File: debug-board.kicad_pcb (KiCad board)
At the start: 2 copper layers, 10 parts, among them P1 CONN_01X04, P2 CONN_01X01

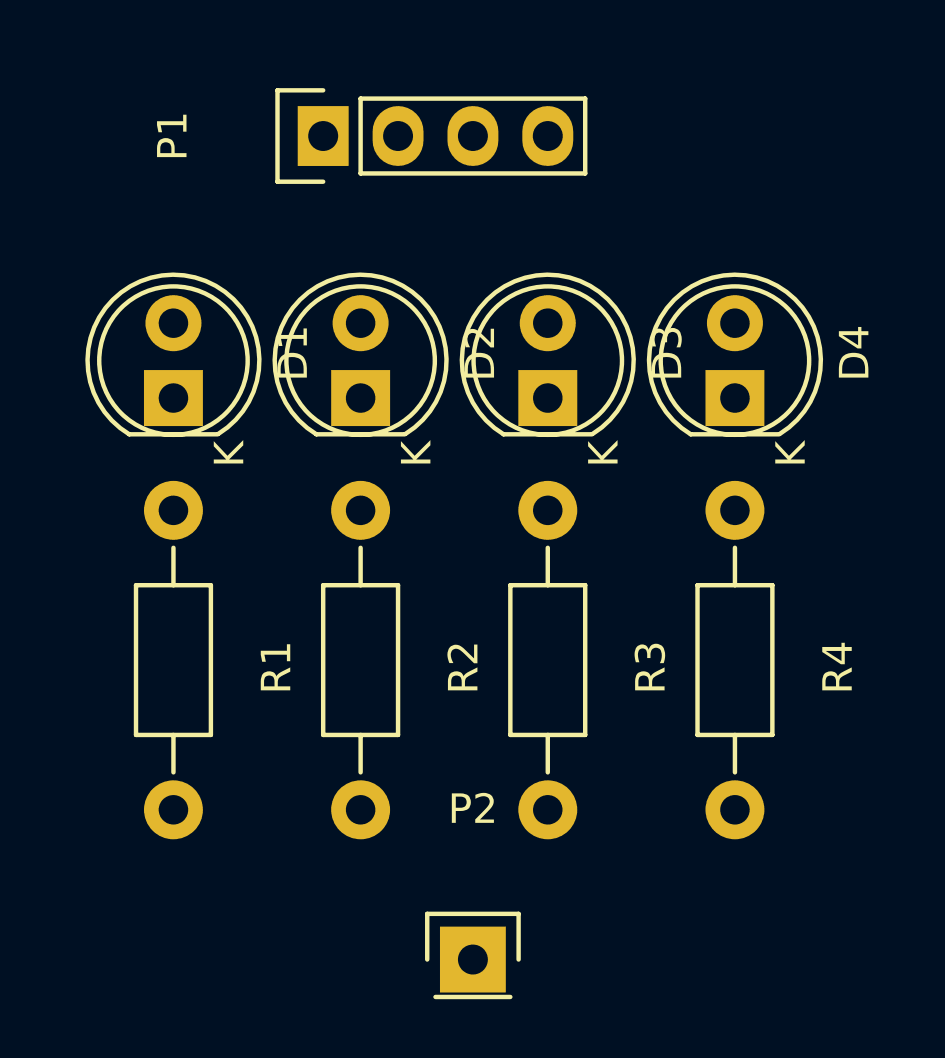
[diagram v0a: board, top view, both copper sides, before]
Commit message: Layout PCB.
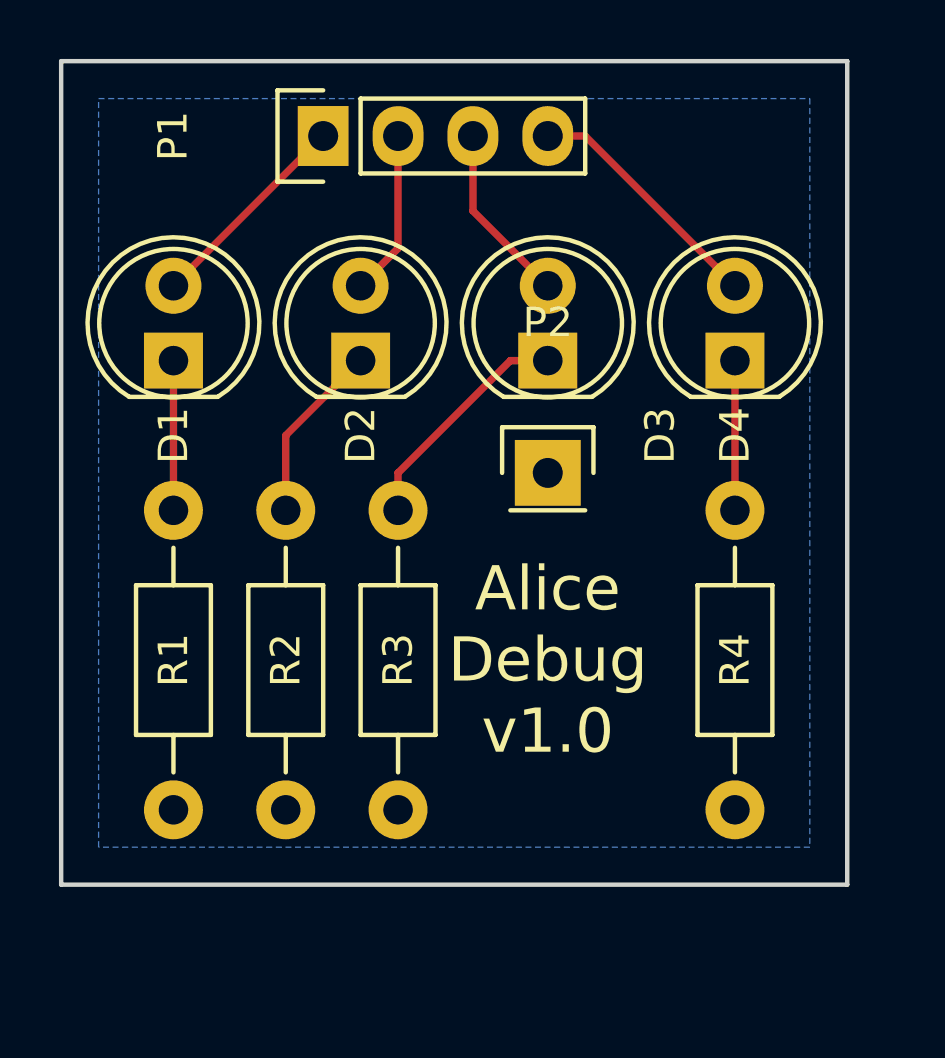
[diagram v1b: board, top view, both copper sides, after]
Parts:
- moved P2 16.7 mm to (151.1, 101.6)
- moved R3 5.08 mm to (146.1, 108.0)
- moved R2 2.54 mm to (142.2, 108.0)
- moved D1 1.27 mm to (138.4, 97.8)
- moved D2 1.27 mm to (144.8, 97.8)
- moved D3 1.27 mm to (151.1, 97.8)
- moved D4 1.27 mm to (157.5, 97.8)
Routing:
- net Net-(D4-Pad2): track 0.00 -> 8.45 mm
- net Net-(D3-Pad1): track 0.00 -> 7.93 mm
- net Net-(D1-Pad2): track 0.00 -> 7.18 mm
- net Net-(D2-Pad1): track 0.00 -> 6.13 mm
- net Net-(D3-Pad2): track 0.00 -> 6.13 mm
- net Net-(D2-Pad2): track 0.00 -> 5.61 mm
- net Net-(D4-Pad1): track 0.00 -> 5.08 mm
- net Net-(D1-Pad1): track 0.00 -> 5.08 mm
- added copper zone on B.Cu, net GND
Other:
- board outline added: 26.7 x 27.9 mm
- board text added: "Alice Debug v1.0"
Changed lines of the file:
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@@
   (general
     (links 12)
-    (no_connects 12)
+    (no_connects 0)
     (area 0 0 0 0)
     (thickness 1.6)
-    (drawings 0)
-    (tracks 0)
+    (drawings 5)
+    (tracks 14)
     (zones 0)
     (modules 10)
@@
   )
   (module LEDs:LED-5MM (layer F.Cu)
-    (at 138.43 99.06 90)
+    (at 138.43 97.79 90)
     (descr "LED 5mm round vertical")
     (tags "LED 5mm round vertical")
-    (fp_text reference D1 (at 1.524 4.064 90) (layer F.SilkS)
-      (effects (font (size 1 1) (thickness 0.15)))
-    )
-    (fp_text value LED (at 1.524 -3.937 90) (layer F.Fab)
+    (fp_text reference D1 (at -2.54 0 90) (layer F.SilkS)
+      (effects (font (size 1 1) (thickness 0.15)))
+    )
+    (fp_text value LED (at 1.524 -3.937 90) (layer F.Fab) hide
       (effects (font (size 1 1) (thickness 0.15)))
     )
@@
     (fp_line (start -1.23 1.5) (end -1.23 -1.5) (layer F.SilkS) (width 0.15))
     (fp_circle (center 1.27 0) (end 0.97 -2.5) (layer F.SilkS) (width 0.15))
-    (fp_text user K (at -1.905 1.905 90) (layer F.SilkS)
-      (effects (font (size 1 1) (thickness 0.15)))
-    )
     (pad 1 thru_hole rect (at 0 0 180) (size 2 1.9) (drill 1.00076) (layers *.Cu *.Mask F.SilkS)
       (net 1 "Net-(D1-Pad1)"))
@@
   )
   (module LEDs:LED-5MM (layer F.Cu)
-    (at 144.78 99.06 90)
+    (at 144.78 97.79 90)
     (descr "LED 5mm round vertical")
     (tags "LED 5mm round vertical")
-    (fp_text reference D2 (at 1.524 4.064 90) (layer F.SilkS)
-      (effects (font (size 1 1) (thickness 0.15)))
-    )
-    (fp_text value LED (at 1.524 -3.937 90) (layer F.Fab)
+    (fp_text reference D2 (at -2.54 0 90) (layer F.SilkS)
+      (effects (font (size 1 1) (thickness 0.15)))
+    )
+    (fp_text value LED (at 1.524 -3.937 90) (layer F.Fab) hide
       (effects (font (size 1 1) (thickness 0.15)))
     )
@@
     (fp_line (start -1.23 1.5) (end -1.23 -1.5) (layer F.SilkS) (width 0.15))
     (fp_circle (center 1.27 0) (end 0.97 -2.5) (layer F.SilkS) (width 0.15))
-    (fp_text user K (at -1.905 1.905 90) (layer F.SilkS)
-      (effects (font (size 1 1) (thickness 0.15)))
-    )
     (pad 1 thru_hole rect (at 0 0 180) (size 2 1.9) (drill 1.00076) (layers *.Cu *.Mask F.SilkS)
       (net 3 "Net-(D2-Pad1)"))
@@
   )
   (module LEDs:LED-5MM (layer F.Cu)
-    (at 151.13 99.06 90)
+    (at 151.13 97.79 90)
     (descr "LED 5mm round vertical")
     (tags "LED 5mm round vertical")
-    (fp_text reference D3 (at 1.524 4.064 90) (layer F.SilkS)
-      (effects (font (size 1 1) (thickness 0.15)))
-    )
-    (fp_text value LED (at 1.524 -3.937 90) (layer F.Fab)
+    (fp_text reference D3 (at -2.54 3.81 90) (layer F.SilkS)
+      (effects (font (size 1 1) (thickness 0.15)))
+    )
+    (fp_text value LED (at 1.524 -3.937 90) (layer F.Fab) hide
       (effects (font (size 1 1) (thickness 0.15)))
     )
@@
     (fp_line (start -1.23 1.5) (end -1.23 -1.5) (layer F.SilkS) (width 0.15))
     (fp_circle (center 1.27 0) (end 0.97 -2.5) (layer F.SilkS) (width 0.15))
-    (fp_text user K (at -1.905 1.905 90) (layer F.SilkS)
-      (effects (font (size 1 1) (thickness 0.15)))
-    )
     (pad 1 thru_hole rect (at 0 0 180) (size 2 1.9) (drill 1.00076) (layers *.Cu *.Mask F.SilkS)
       (net 5 "Net-(D3-Pad1)"))
@@
   )
   (module LEDs:LED-5MM (layer F.Cu)
-    (at 157.48 99.06 90)
+    (at 157.48 97.79 90)
     (descr "LED 5mm round vertical")
     (tags "LED 5mm round vertical")
-    (fp_text reference D4 (at 1.524 4.064 90) (layer F.SilkS)
-      (effects (font (size 1 1) (thickness 0.15)))
-    )
-    (fp_text value LED (at 1.524 -3.937 90) (layer F.Fab)
+    (fp_text reference D4 (at -2.54 0 90) (layer F.SilkS)
+      (effects (font (size 1 1) (thickness 0.15)))
+    )
+    (fp_text value LED (at 1.524 -3.937 90) (layer F.Fab) hide
       (effects (font (size 1 1) (thickness 0.15)))
     )
@@
     (fp_line (start -1.23 1.5) (end -1.23 -1.5) (layer F.SilkS) (width 0.15))
     (fp_circle (center 1.27 0) (end 0.97 -2.5) (layer F.SilkS) (width 0.15))
-    (fp_text user K (at -1.905 1.905 90) (layer F.SilkS)
-      (effects (font (size 1 1) (thickness 0.15)))
-    )
     (pad 1 thru_hole rect (at 0 0 180) (size 2 1.9) (drill 1.00076) (layers *.Cu *.Mask F.SilkS)
       (net 7 "Net-(D4-Pad1)"))
@@
       (effects (font (size 1 1) (thickness 0.15)))
     )
-    (fp_text value CONN_01X04 (at 0 -3.1 90) (layer F.Fab)
+    (fp_text value CONN_01X04 (at 0 -3.1 90) (layer F.Fab) hide
       (effects (font (size 1 1) (thickness 0.15)))
     )
@@
   )
   (module Pin_Headers:Pin_Header_Straight_1x01 (layer F.Cu)
-    (at 148.59 118.11)
+    (at 151.13 101.6)
     (descr "Through hole pin header")
     (tags "pin header")
@@
       (effects (font (size 1 1) (thickness 0.15)))
     )
-    (fp_text value CONN_01X01 (at 0 -3.1) (layer F.Fab)
+    (fp_text value CONN_01X01 (at 0 -3.1) (layer F.Fab) hide
       (effects (font (size 1 1) (thickness 0.15)))
     )
@@
     (descr "Resistor, Axial,  RM 10mm, 1/3W,")
     (tags "Resistor, Axial, RM 10mm, 1/3W,")
-    (fp_text reference R1 (at 0.24892 -3.50012 270) (layer F.SilkS)
-      (effects (font (size 1 1) (thickness 0.15)))
-    )
-    (fp_text value 220 (at 3.81 3.81 270) (layer F.Fab)
+    (fp_text reference R1 (at 0 0 270) (layer F.SilkS)
+      (effects (font (size 1 1) (thickness 0.15)))
+    )
+    (fp_text value 220 (at 3.81 3.81 270) (layer F.Fab) hide
       (effects (font (size 1 1) (thickness 0.15)))
     )
@@
   )
   (module Resistors_ThroughHole:Resistor_Horizontal_RM10mm (layer F.Cu)
-    (at 144.78 107.95 270)
+    (at 142.24 107.95 270)
     (descr "Resistor, Axial,  RM 10mm, 1/3W,")
     (tags "Resistor, Axial, RM 10mm, 1/3W,")
-    (fp_text reference R2 (at 0.24892 -3.50012 270) (layer F.SilkS)
-      (effects (font (size 1 1) (thickness 0.15)))
-    )
-    (fp_text value 220 (at 3.81 3.81 270) (layer F.Fab)
+    (fp_text reference R2 (at 0 0 270) (layer F.SilkS)
+      (effects (font (size 1 1) (thickness 0.15)))
+    )
+    (fp_text value 220 (at 3.81 3.81 270) (layer F.Fab) hide
       (effects (font (size 1 1) (thickness 0.15)))
     )
@@
   )
   (module Resistors_ThroughHole:Resistor_Horizontal_RM10mm (layer F.Cu)
-    (at 151.13 107.95 270)
+    (at 146.05 107.95 270)
     (descr "Resistor, Axial,  RM 10mm, 1/3W,")
     (tags "Resistor, Axial, RM 10mm, 1/3W,")
-    (fp_text reference R3 (at 0.24892 -3.50012 270) (layer F.SilkS)
-      (effects (font (size 1 1) (thickness 0.15)))
-    )
-    (fp_text value 220 (at 3.81 3.81 270) (layer F.Fab)
+    (fp_text reference R3 (at 0 0 270) (layer F.SilkS)
+      (effects (font (size 1 1) (thickness 0.15)))
+    )
+    (fp_text value 220 (at 3.81 3.81 270) (layer F.Fab) hide
       (effects (font (size 1 1) (thickness 0.15)))
     )
@@
     (descr "Resistor, Axial,  RM 10mm, 1/3W,")
     (tags "Resistor, Axial, RM 10mm, 1/3W,")
-    (fp_text reference R4 (at 0.24892 -3.50012 270) (layer F.SilkS)
-      (effects (font (size 1 1) (thickness 0.15)))
-    )
-    (fp_text value 220 (at 3.81 3.81 270) (layer F.Fab)
+    (fp_text reference R4 (at 0 0 270) (layer F.SilkS)
+      (effects (font (size 1 1) (thickness 0.15)))
+    )
+    (fp_text value 220 (at 3.81 3.81 270) (layer F.Fab) hide
       (effects (font (size 1 1) (thickness 0.15)))
     )
@@
     )
   )
+  (gr_text "Alice\nDebug\nv1.0" (at 151.13 107.95) (layer F.SilkS)
+    (effects (font (size 1.5 1.5) (thickness 0.3)))
+  )
+  (gr_line (start 134.62 115.57) (end 134.62 87.63) (angle 90) (layer Edge.Cuts) (width 0.15))
+  (gr_line (start 161.29 115.57) (end 134.62 115.57) (angle 90) (layer Edge.Cuts) (width 0.15))
+  (gr_line (start 161.29 87.63) (end 161.29 115.57) (angle 90) (layer Edge.Cuts) (width 0.15))
+  (gr_line (start 134.62 87.63) (end 161.29 87.63) (angle 90) (layer Edge.Cuts) (width 0.15))
+  (segment (start 138.43 102.87) (end 138.43 97.79) (width 0.25) (layer F.Cu) (net 1))
+  (segment (start 143.51 90.17) (end 138.43 95.25) (width 0.25) (layer F.Cu) (net 2))
+  (segment (start 142.24 102.87) (end 142.24 100.33) (width 0.25) (layer F.Cu) (net 3))
+  (segment (start 142.24 100.33) (end 144.78 97.79) (width 0.25) (layer F.Cu) (net 3))
+  (segment (start 146.05 90.17) (end 146.05 93.98) (width 0.25) (layer F.Cu) (net 4))
+  (segment (start 146.05 93.98) (end 144.78 95.25) (width 0.25) (layer F.Cu) (net 4))
+  (segment (start 146.05 102.87) (end 146.05 101.6) (width 0.25) (layer F.Cu) (net 5))
+  (segment (start 149.86 97.79) (end 151.13 97.79) (width 0.25) (layer F.Cu) (net 5))
+  (segment (start 146.05 101.6) (end 149.86 97.79) (width 0.25) (layer F.Cu) (net 5))
+  (segment (start 148.59 90.17) (end 148.59 92.71) (width 0.25) (layer F.Cu) (net 6))
+  (segment (start 148.59 92.71) (end 151.13 95.25) (width 0.25) (layer F.Cu) (net 6))
+  (segment (start 157.48 102.87) (end 157.48 97.79) (width 0.25) (layer F.Cu) (net 7))
+  (segment (start 151.13 90.17) (end 152.4 90.17) (width 0.25) (layer F.Cu) (net 8))
+  (segment (start 152.4 90.17) (end 157.48 95.25) (width 0.25) (layer F.Cu) (net 8))
+  (zone (net 9) (net_name GND) (layer B.Cu) (hatch edge 0.508)
+    (connect_pads (clearance 0.508))
+    (min_thickness 0.254)
+    (fill yes (arc_segments 16) (thermal_gap 0.508) (thermal_bridge_width 0.508))
+    (polygon
+      (pts
+        (xy 160.02 114.3) (xy 135.89 114.3) (xy 135.89 88.9) (xy 160.02 88.9) (xy 160.02 114.3)
+      )
+    )
+  )
